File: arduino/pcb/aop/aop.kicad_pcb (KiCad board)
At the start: 2 copper layers, 45 x 55 mm, 22 parts, among them Q1 AO4435, SW1 SW_Push, SW2 SW_Push, U1 ESP32-C3_SUPERMINI_TH, U2 DS3231M

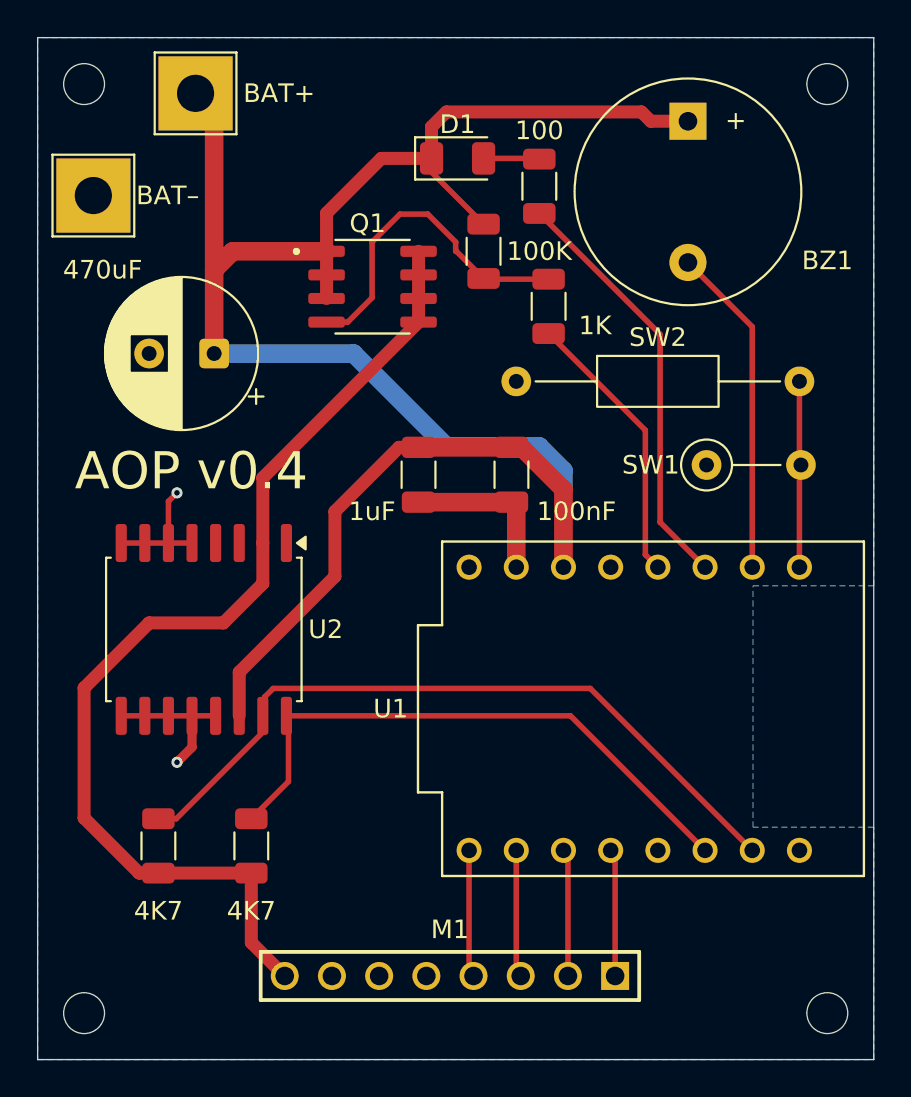
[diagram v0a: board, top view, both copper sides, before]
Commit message: [pcb] Send v0.4 for fabrication
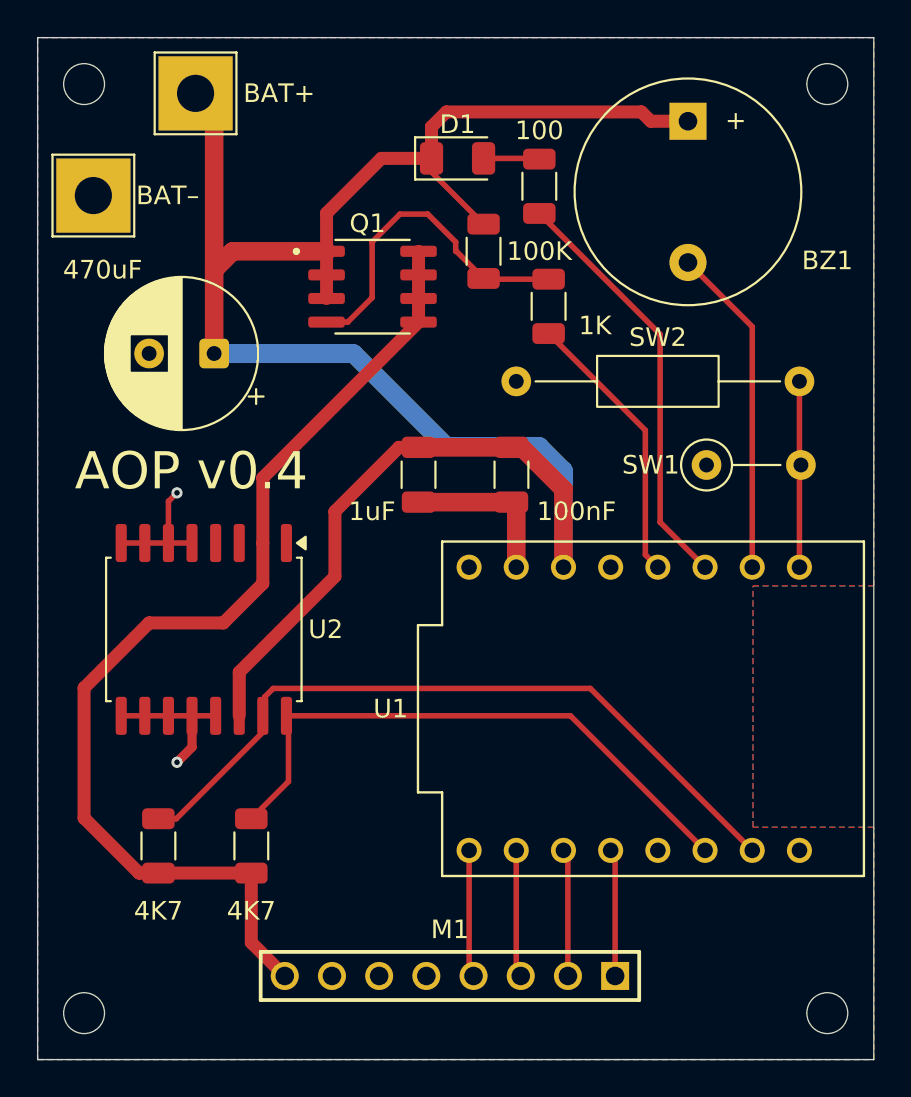
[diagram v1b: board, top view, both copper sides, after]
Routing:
- added copper zone on F.Cu, net GND
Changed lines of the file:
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@@
 	(zone
 		(net "GND")
-		(layer "B.Cu")
+		(layers "F.Cu" "B.Cu")
 		(hatch edge 0.5)
 		(connect_pads
